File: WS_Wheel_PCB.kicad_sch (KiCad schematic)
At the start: 5 parts, among them U1 Teensy4.1

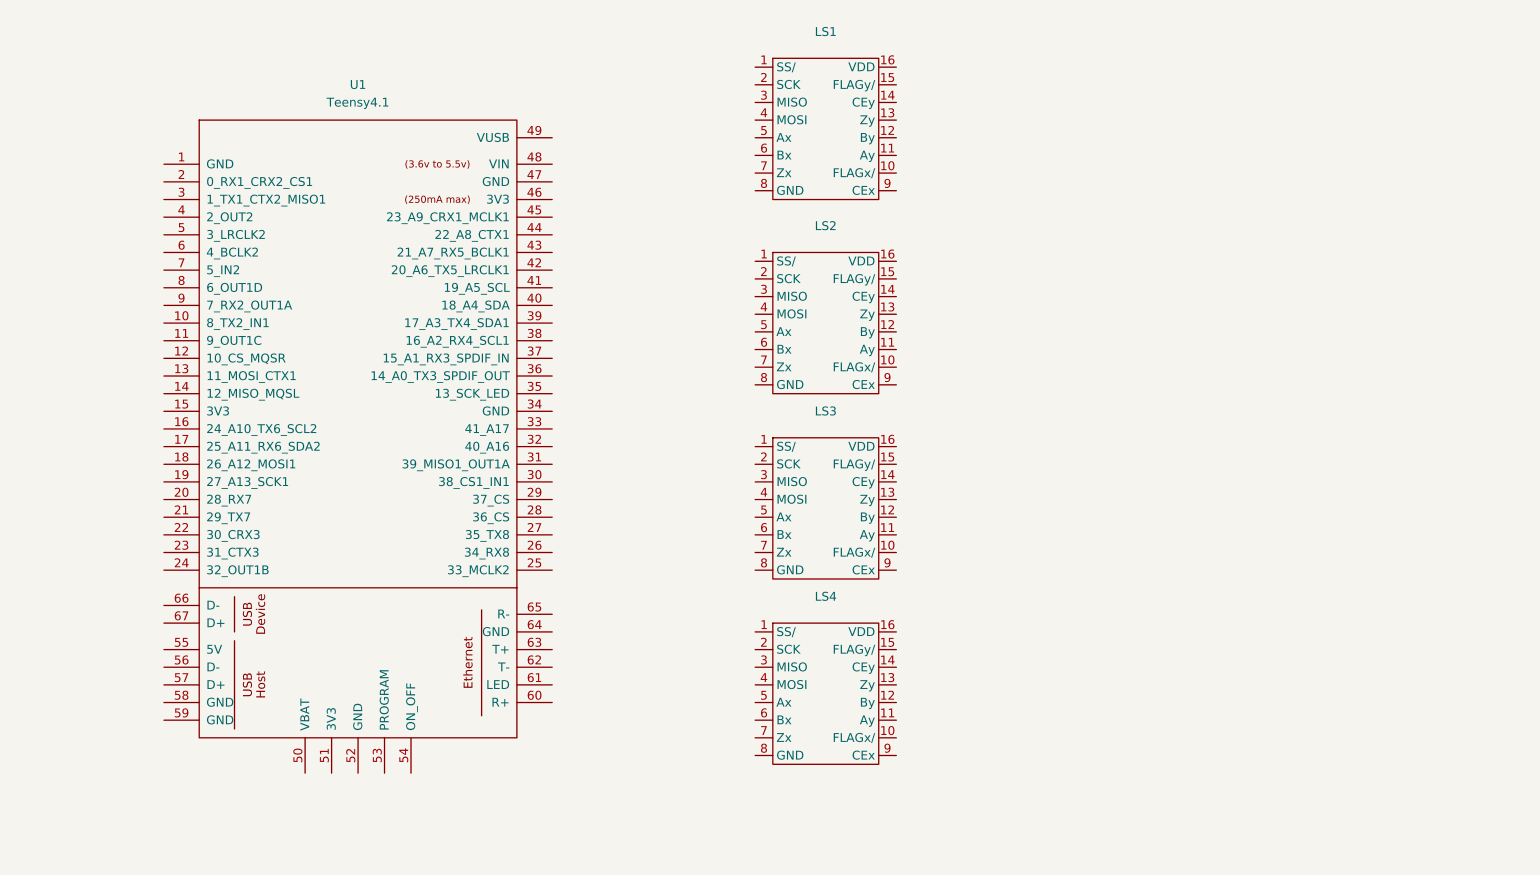
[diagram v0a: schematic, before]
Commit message: Saving for the day
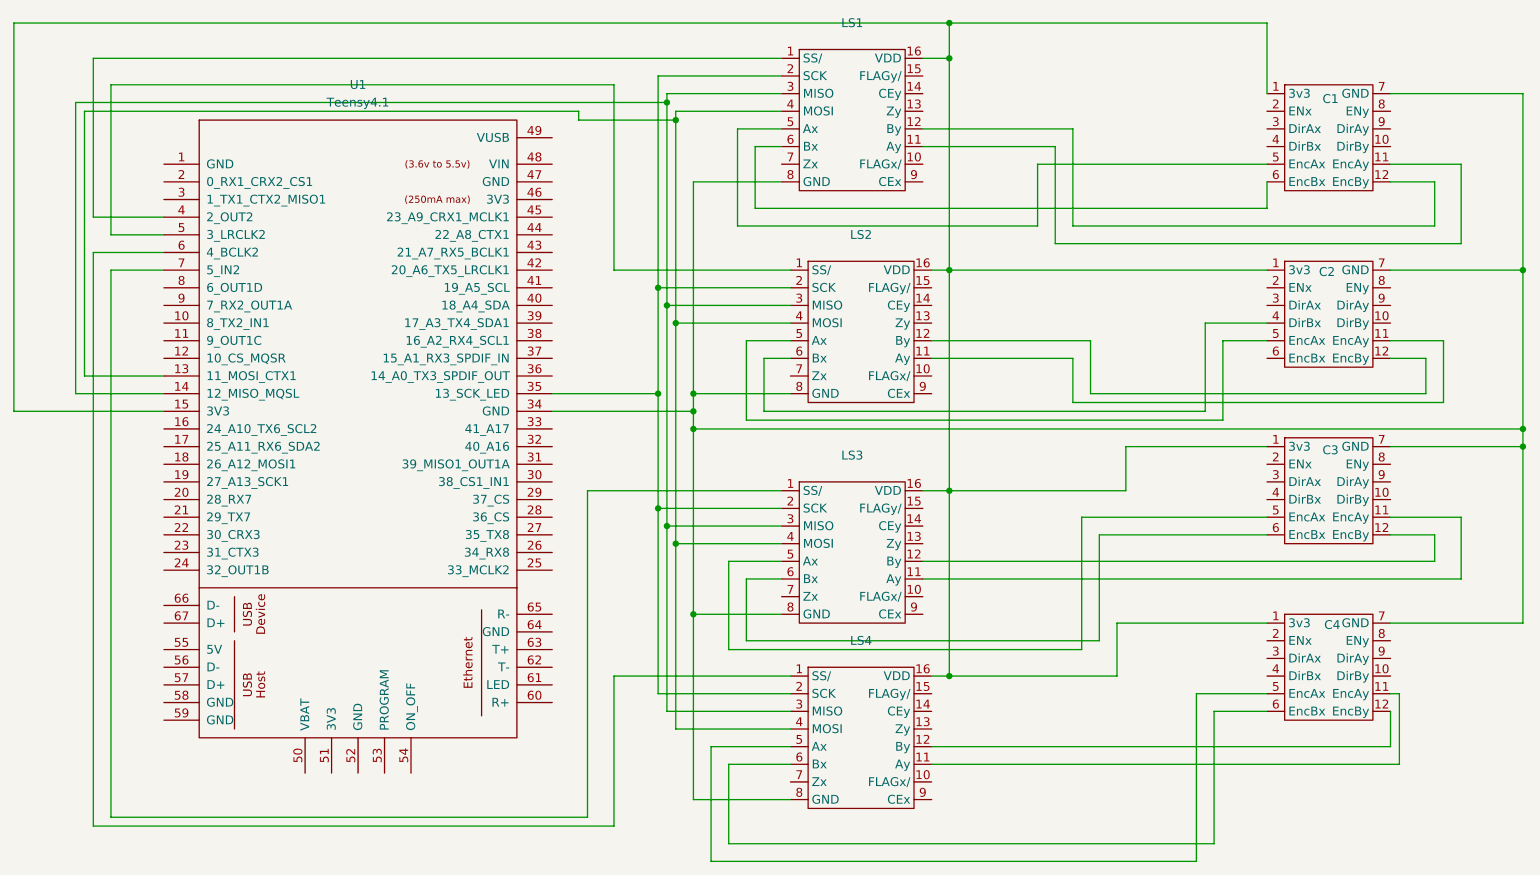
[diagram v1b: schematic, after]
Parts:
- added C1, C2, C3, C4: ~, Connector_Molex:Molex_Nano-Fit_105310-xx12_2x06_P2.50mm_Vertical, symbol custom_components:Motor_Conn
- LS1, LS2, LS3, LS4: footprint (none) -> Custom_Components:LS7466
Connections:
- net at LS3.1 (SS/): now also U1.7 (5_IN2)
- net at LS3.11 (Ay): now also C3.11 (EncAy)
- net at LS3.12 (By): now also C3.12 (EncBy)
- net at LS3.16 (VDD): now also LS1.16 (VDD), LS2.16 (VDD), LS4.16 (VDD), U1.15 (3V3), C1.1 (3v3), C2.1 (3v3), C3.1 (3v3), C4.1 (3v3)
- net at LS3.2 (SCK): now also LS1.2 (SCK), LS2.2 (SCK), LS4.2 (SCK), U1.35 (13_SCK_LED)
- net at LS3.3 (MISO): now also LS1.3 (MISO), LS2.3 (MISO), LS4.3 (MISO), U1.14 (12_MISO_MQSL)
- net at LS3.4 (MOSI): now also LS1.4 (MOSI), LS2.4 (MOSI), LS4.4 (MOSI), U1.13 (11_MOSI_CTX1)
- net at LS3.5 (Ax): now also C3.5 (EncAx)
- net at LS3.6 (Bx): now also C3.6 (EncBx)
- net at LS3.8 (GND): now also LS1.8 (GND), LS2.8 (GND), LS4.8 (GND), U1.34 (GND), C1.7 (GND), C2.7 (GND), C3.7 (GND), C4.7 (GND)
- net at LS4.1 (SS/): now also U1.6 (4_BCLK2)
- net at LS4.11 (Ay): now also C4.11 (EncAy)
- net at LS4.12 (By): now also C4.12 (EncBy)
- net at LS4.5 (Ax): now also C4.5 (EncAx)
- net at LS4.6 (Bx): now also C4.6 (EncBx)
- net at LS2.1 (SS/): now also U1.5 (3_LRCLK2)
- net at LS2.11 (Ay): now also C2.11 (EncAy)
- net at LS2.12 (By): now also C2.12 (EncBy)
- net at LS2.5 (Ax): now also C2.5 (EncAx)
- net at LS2.6 (Bx): now also C2.4 (DirBx)
- net at U1.4 (2_OUT2): now also LS1.1 (SS/)
- net at LS1.11 (Ay): now also C1.11 (EncAy)
- net at LS1.12 (By): now also C1.12 (EncBy)
- net at LS1.5 (Ax): now also C1.5 (EncAx)
- net at LS1.6 (Bx): now also C1.6 (EncBx)
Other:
- moved on the sheet: LS1, LS2, LS3, LS4

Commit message: Final?
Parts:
- added Enc1, Enc2: ~, symbol custom_components:Quadrature_Encoder
- added J1: 5V in, Connector_Molex:Molex_Nano-Fit_105309-xx02_1x02_P2.50mm_Vertical, symbol Connector:Conn_01x02_Pin
- added M1, M2: Motor_DC, symbol Motor:Motor_DC
- added U2: ~, symbol custom_components:Motor_Conn
- added U3: ~, symbol custom_components:MotorDriver
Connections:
- net at C2.10 (DirBy): now also U1.18 (26_A12_MOSI1)
- net at C2.2 (ENx): now also U1.42 (20_A6_TX5_LRCLK1)
- net at C2.3 (DirAx): now also U1.41 (19_A5_SCL)
- net at C2.4 (DirBx): now also U1.40 (18_A4_SDA); no longer LS2.6 (Bx)
- net at C2.6 (EncBx): now also LS2.6 (Bx)
- net at C2.8 (ENy): now also U1.16 (24_A10_TX6_SCL2)
- net at C2.9 (DirAy): now also U1.17 (25_A11_RX6_SDA2)
- net at C3.10 (DirBy): now also U1.21 (29_TX7)
- net at C3.2 (ENx): now also U1.39 (17_A3_TX4_SDA1)
- net at C3.3 (DirAx): now also U1.38 (16_A2_RX4_SCL1)
- net at C3.4 (DirBx): now also U1.30 (38_CS1_IN1)
- net at C3.8 (ENy): now also U1.19 (27_A13_SCK1)
- net at C3.9 (DirAy): now also U1.20 (28_RX7)
- net at C1.10 (DirBy): now also U1.10 (8_TX2_IN1)
- net at C1.2 (ENx): now also U1.45 (23_A9_CRX1_MCLK1)
- net at C1.3 (DirAx): now also U1.44 (22_A8_CTX1)
- net at C1.4 (DirBx): now also U1.43 (21_A7_RX5_BCLK1)
- net at C1.8 (ENy): now also U1.8 (6_OUT1D)
- net at C1.9 (DirAy): now also U1.9 (7_RX2_OUT1A)
- net at U1.22 (30_CRX3): now also C4.8 (ENy)
- net at U1.23 (31_CTX3): now also C4.9 (DirAy)
- net at U1.24 (32_OUT1B): now also C4.10 (DirBy)
- net at U1.31 (39_MISO1_OUT1A): now also C4.4 (DirBx)
- net at U1.32 (40_A16): now also C4.3 (DirAx)
- net at U1.33 (41_A17): now also C4.2 (ENx)
- net at U1.47 (GND): now also J1.1 (Pin_1)
- net at U1.48 (VIN): now also J1.2 (Pin_2)
- new net: M2.1 (+), U3. (V_motor)
- new net: M2.2 (-), U3. (V_motor)
- new net: M1.1 (+), U3. (V_motor)
- new net: M1.2 (-), U3. (V_motor)
- new net: Enc1.1 (Vin), U2.1 (3v3), U3.1 (Vcc)
- new net: Enc2.4 (GND), U3.10 (GND)
- new net: U2.2 (ENx), U3.2 (P1)
- new net: U2.3 (DirAx), U3.3 (A1)
- new net: U2.4 (DirBx), U3.4 (B1)
- new net: Enc1.4 (GND), U2.7 (GND), U3.5 (GND)
- new net: Enc2.1 (Vin), U3.6 (Vcc)
- new net: U2.8 (ENy), U3.7 (P2)
- new net: U2.9 (DirAy), U3.8 (A2)
- new net: U2.10 (DirBy), U3.9 (B2)
- new net: Enc2.2 (A), U2.12 (EncBy)
- new net: Enc2.3 (B), U2.11 (EncAy)
- new net: Enc1.2 (A), U2.5 (EncAx)
- new net: Enc1.3 (B), U2.6 (EncBx)
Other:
- added sheet WiringHarness (harness.kicad_sch)
- note added: "Wheel PCB Connector Output"
- moved on the sheet: C1, C2, C3, C4, LS1, LS2, LS3, LS4, U1
